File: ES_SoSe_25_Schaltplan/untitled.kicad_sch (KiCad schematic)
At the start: 9 parts, among them M1 Motor_DC, M2 Motor_Servo, U6 L298N

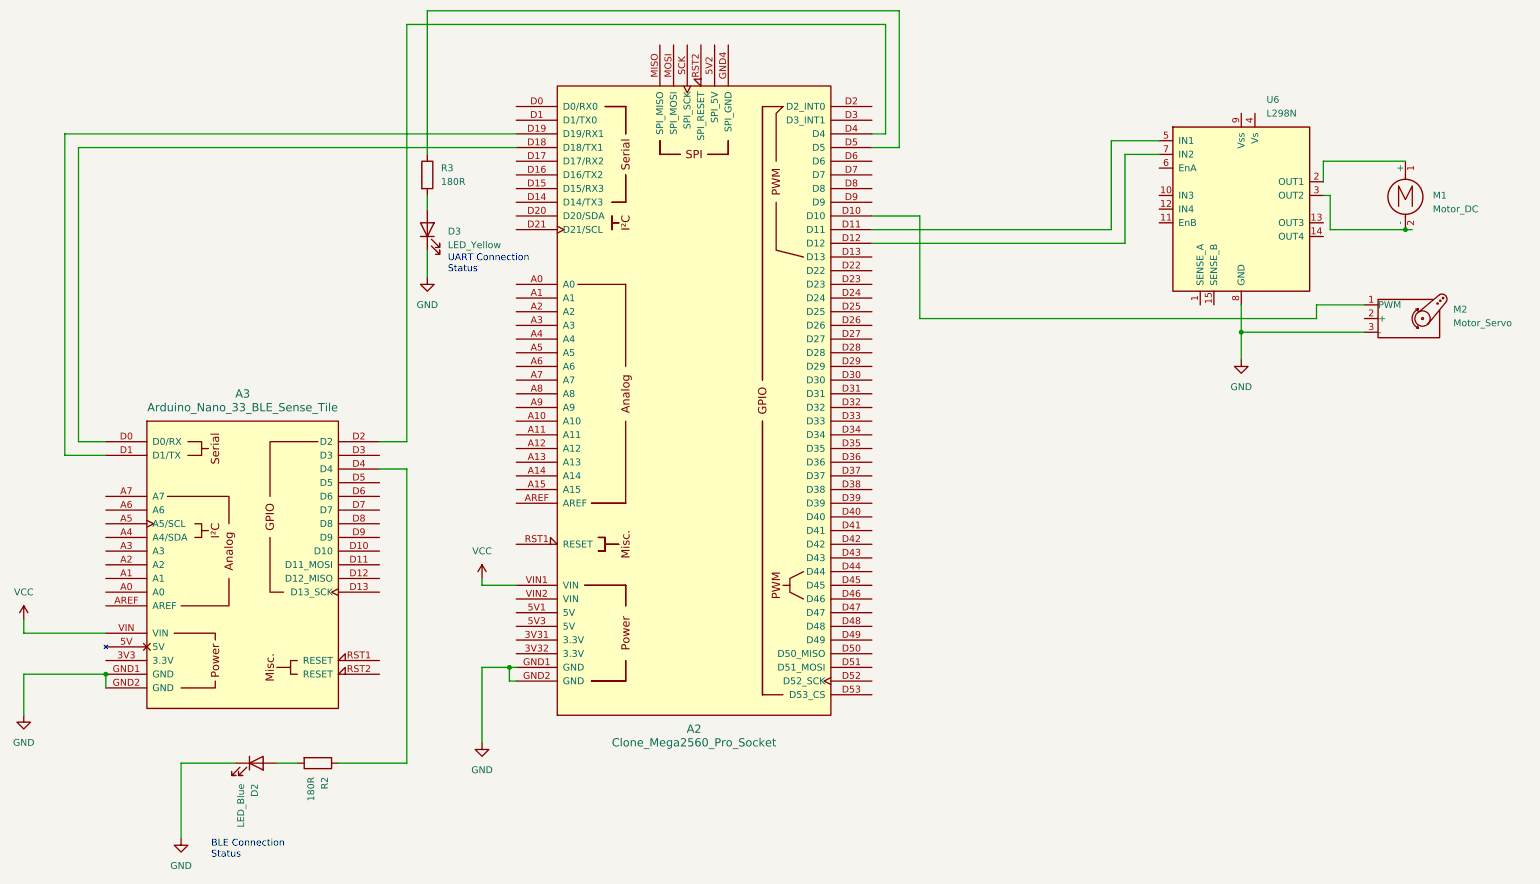
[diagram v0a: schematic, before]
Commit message: Schaltplan Vollständig Jan
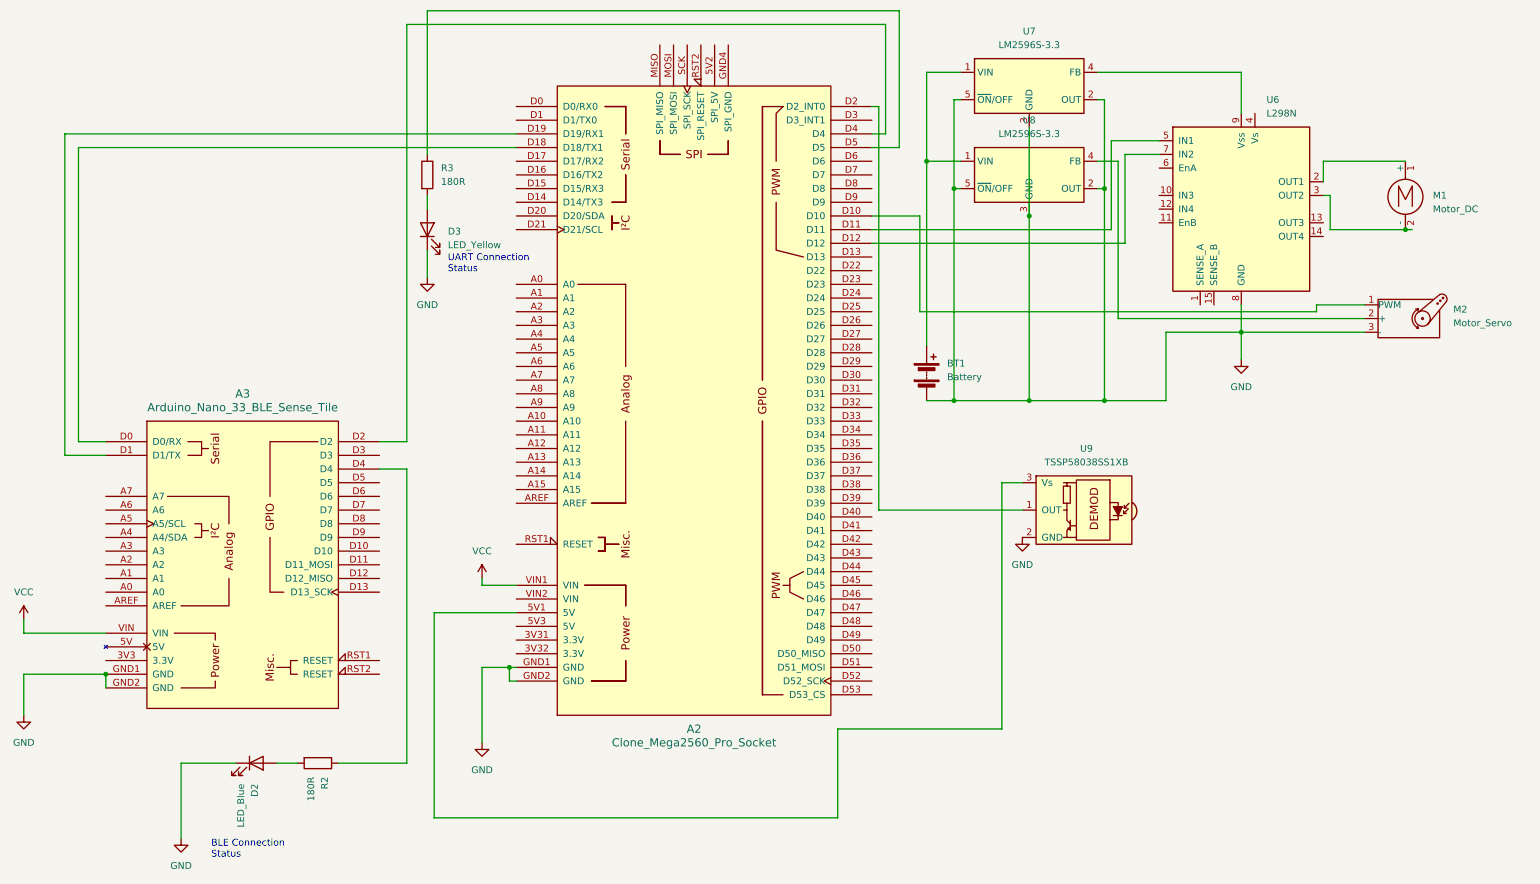
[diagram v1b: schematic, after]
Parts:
- added BT1: Battery, symbol Device:Battery
- added U7, U8: LM2596S-3.3, Package_TO_SOT_SMD:TO-263-5_TabPin3, symbol Regulator_Switching:LM2596S-3.3
- added U9: TSSP58038SS1XB, OptoDevice:Vishay_MINICAST-3Pin, symbol Sensor_Proximity:TSSP58038SS1XB
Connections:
- net GND: now also BT1.2 (-), U7.2 (OUT), U7.3 (GND), U7.5 (~{ON}/OFF), U8.2 (OUT), U8.3 (GND), U8.5 (~{ON}/OFF), U9.2 (GND)
- net at A2.5V1 (5V): now also U9.3 (Vs)
- net at A2.D2 (D2_INT0): now also U9.1 (OUT)
- net at M2.2 (+): now also U8.4 (FB)
- net at U6.9 (Vss): now also U7.4 (FB)
- new net: BT1.1 (+), U7.1 (VIN), U8.1 (VIN)
